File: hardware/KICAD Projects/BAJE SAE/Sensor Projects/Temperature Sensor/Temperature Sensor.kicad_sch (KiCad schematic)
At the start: 8 parts, among them J1 +5V, J2 Bypass, U1 BA50JC5T

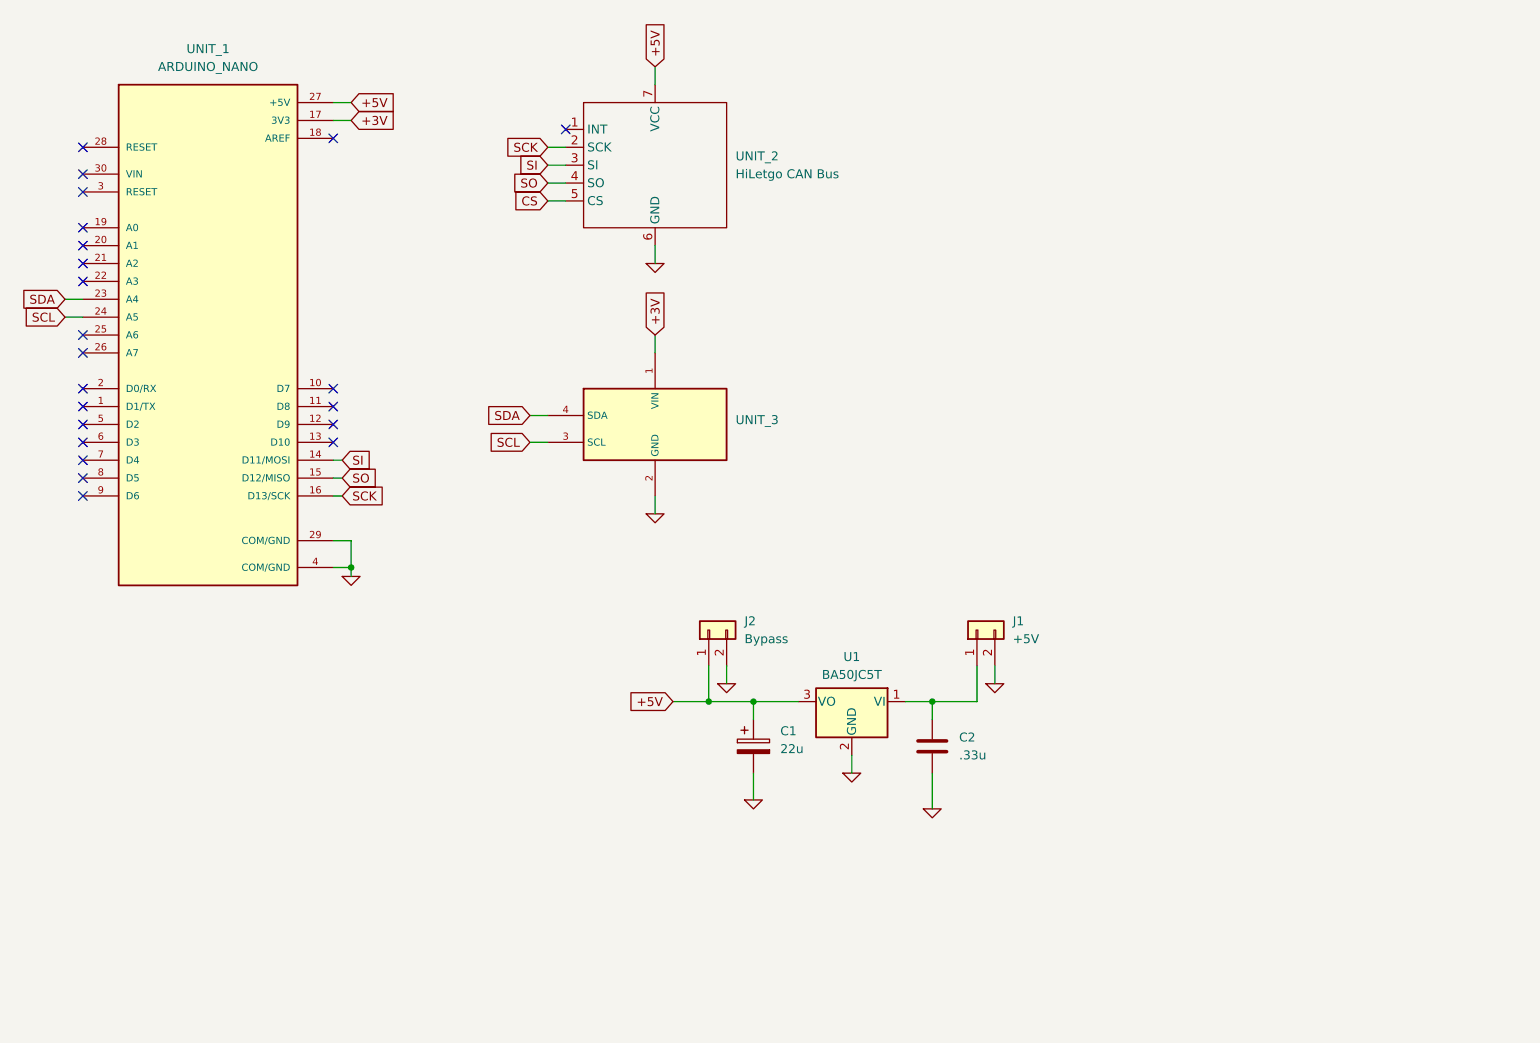
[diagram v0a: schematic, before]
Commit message: Updates to IMU and Temp PCB
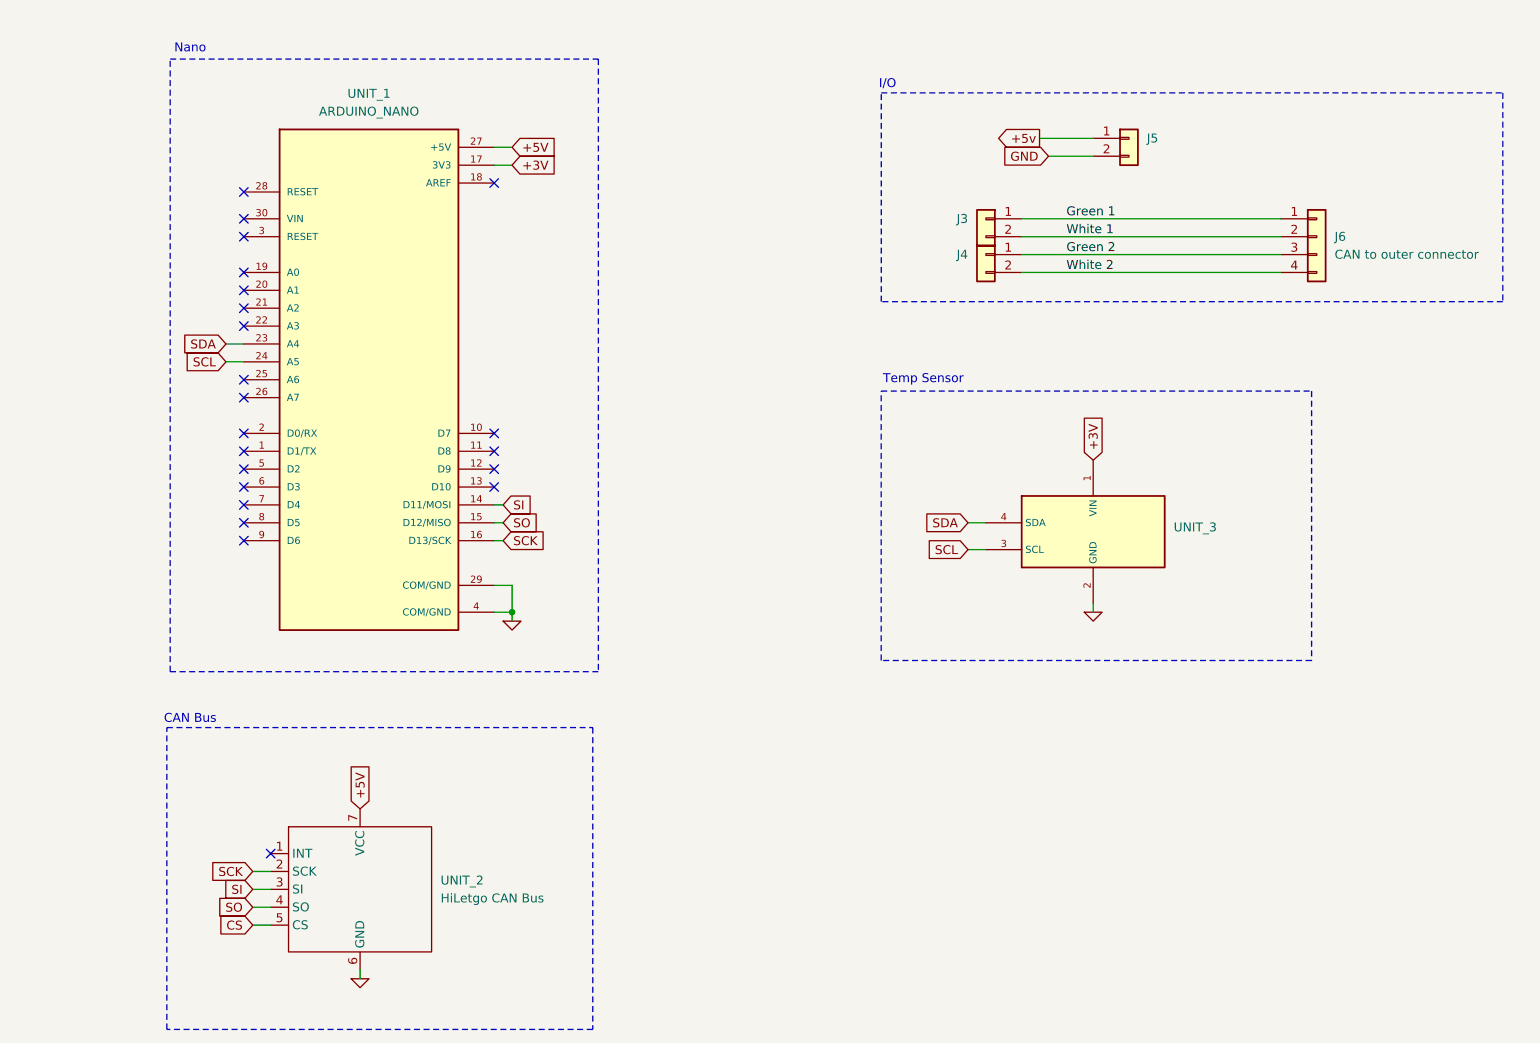
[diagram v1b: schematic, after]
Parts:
- removed C1: 22u, Capacitor_THT:CP_Axial_L11.0mm_D8.0mm_P15.00mm_Horizontal, symbol Device:C_Polarized
- removed C2: .33u, Capacitor_THT:C_Axial_L3.8mm_D2.6mm_P7.50mm_Horizontal, symbol Device:C
- removed J1: +5V, Connector_PinHeader_1.00mm:PinHeader_1x02_P1.00mm_Vertical, symbol Connector_Generic:Conn_01x02
- removed J2: Bypass, Connector_PinHeader_1.00mm:PinHeader_1x02_P1.00mm_Vertical, symbol Connector_Generic:Conn_01x02
- removed U1: BA50JC5T, Package_TO_SOT_THT:TO-220-3_Horizontal_TabDown, symbol Regulator_Linear:LF80_TO220
- added J3, J4: Conn_01x02, Connector_PinHeader_2.54mm:PinHeader_1x02_P2.54mm_Vertical, symbol Connector_Generic:Conn_01x02
- added J5: Conn_01x02, Connector_Wire:SolderWire-0.75sqmm_1x02_P4.8mm_D1.25mm_OD2.3mm_Relief2x, symbol Connector_Generic:Conn_01x02
- added J6: CAN to outer connector, Connector_Wire:SolderWire-0.1sqmm_1x04_P3.6mm_D0.4mm_OD1mm_Relief, symbol Connector_Generic:Conn_01x04
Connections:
- new net +5v: J5.1 (Pin_1)
- new net GND: J5.2 (Pin_2)
- new net Green 1: J3.1 (Pin_1), J6.1 (Pin_1)
- new net Green 2: J4.1 (Pin_1), J6.3 (Pin_3)
- new net White 1: J3.2 (Pin_2), J6.2 (Pin_2)
- new net White 2: J4.2 (Pin_2), J6.4 (Pin_4)
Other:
- note added: "CAN Bus"
- note added: "I/O"
- note added: "Nano"
- note added: "Temp Sensor"
- moved on the sheet: UNIT_1, UNIT_2, UNIT_3
